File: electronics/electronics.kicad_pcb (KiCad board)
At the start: 2 copper layers, 32 x 48.2 mm, 17 parts, among them J1 USB_C_Receptacle_USB2.0_14P, U1 ESP32-S3-WROOM-1, U3 NCP1117-3.3_SOT223, U5 NCP1117-3.3_SOT223

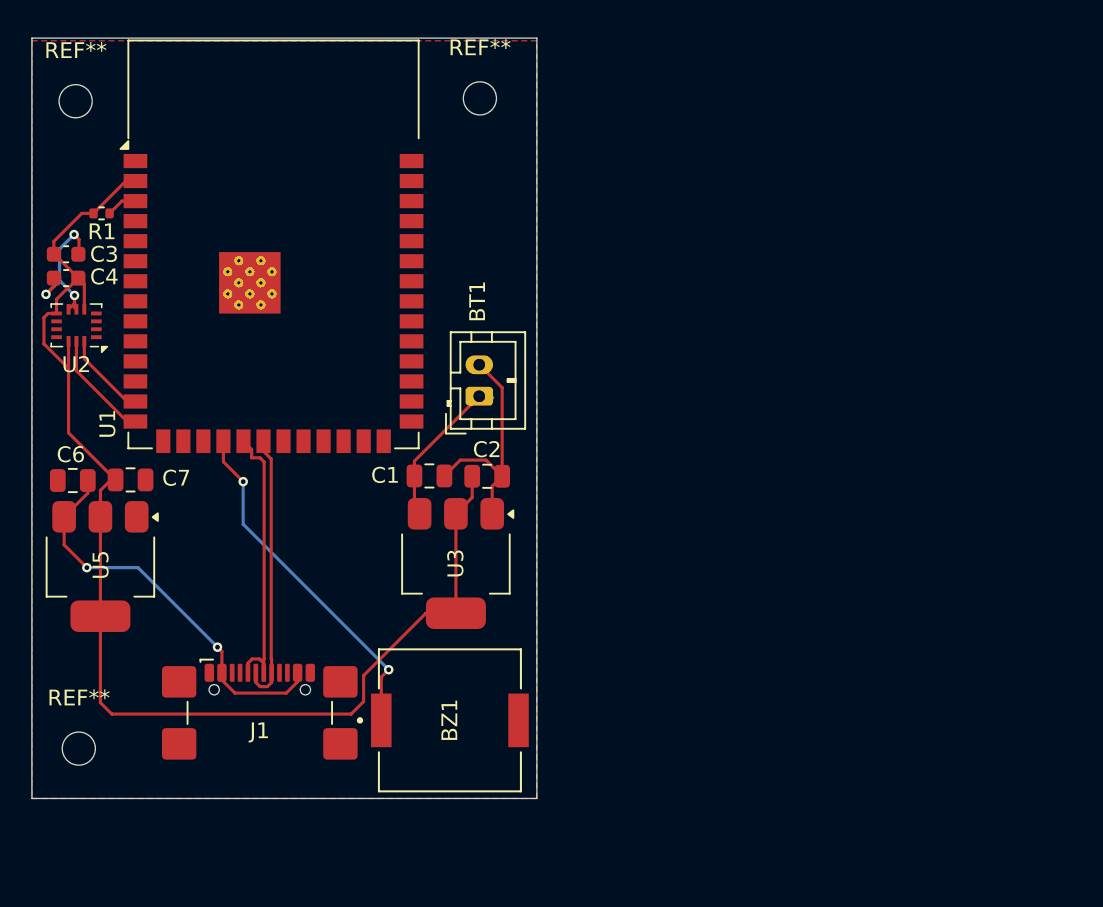
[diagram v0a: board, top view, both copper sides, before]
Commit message: BOM + Gerbers: Final Iteration (Hopefully)
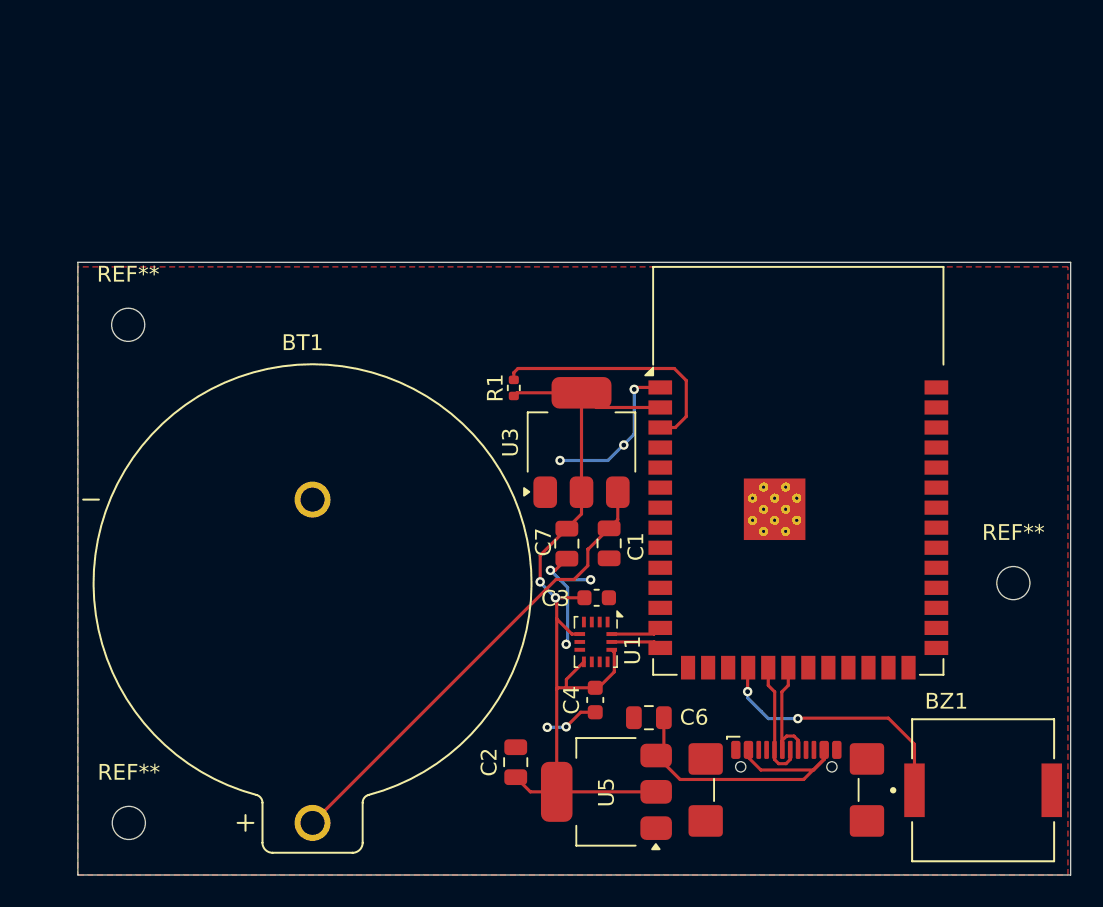
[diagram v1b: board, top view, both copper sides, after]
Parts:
- removed the REF** at (156.1, 75.3)
- removed the REF** at (130.7, 116.5)
- removed the REF** at (130.5, 75.5)
- added REF**: MountingHole_2.1mm, MountingHole:MountingHole_2.1mm, F.Cu at (133.8, 89.7)
- added REF**: MountingHole_2.1mm, MountingHole:MountingHole_2.1mm, F.Cu at (189.9, 106.1)
- added REF**: MountingHole_2.1mm, MountingHole:MountingHole_2.1mm, F.Cu at (133.8, 121.3)
- BT1: footprint Connector_JST:JST_PH_B2B-PH-K_1x02_P2.00mm_Vertical -> Uni:BAT_1025
- BZ1: footprint Global:SPKR_PKMCS0909E4000-R1 -> Uni:SPKR_PKMCS0909E4000-R1
- moved C4 42.9 mm to (163.4, 113.5), turned to -90 degrees
- moved C3 40.1 mm to (163.5, 107.0)
- moved C6 39.5 mm to (166.8, 114.6)
- moved U2 38.5 mm to (163.4, 109.8), turned to -90 degrees
- moved U1 36.2 mm to (176.3, 98.9)
- moved U5 35.1 mm to (164.1, 119.3), turned to 180 degrees
- moved BZ1 34.1 mm to (188.0, 119.2)
- moved J1 33.7 mm to (175.5, 120.3)
- moved R1 28.4 mm to (158.2, 93.7), turned to 90 degrees
- moved C7 27.9 mm to (161.6, 103.6), turned to -90 degrees
- moved C2 18.2 mm to (158.4, 117.4), turned to 90 degrees
- moved BT1 15.9 mm to (145.5, 106.1), turned to 0 degrees
- moved C1 12.2 mm to (164.3, 103.5), turned to -90 degrees
- moved U3 11.1 mm to (162.5, 97.2), turned to 90 degrees
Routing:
- net +3V3: track 79.8 -> 57.2 mm, vias 0 -> 2
- net Net-(BT1-+): track 10.2 -> 29.7 mm
- net Net-(U1-EN): track 1.96 -> 16.0 mm
- net /D-: track 18.0 -> 7.60 mm
- net /D+: track 17.3 -> 7.60 mm
- net /BZR: track 22.4 -> 16.7 mm
- net GND: track 25.9 -> 21.9 mm, vias 3 -> 8
- net Net-(U5-VI): track 25.3 -> 21.5 mm, vias 2 -> 0
- net /SCL: track 6.94 -> 3.23 mm
- net /SDA: track 5.47 -> 3.24 mm
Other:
- board size 32 x 48.2 mm -> 62.9 x 38.8 mm
